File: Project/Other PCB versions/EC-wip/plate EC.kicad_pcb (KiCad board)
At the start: 4 copper layers, 245.7 x 83.6 mm, 154 parts, among them J2 USB_C_Receptacle_USB2.0, SW1 BOOT0, U1 USBLC6-2SC6, U2 XC6206PxxxMR-Regulator_Linear, U3 OPA354, U4 74AHCT1G125, U5 74HC4051, U7 74HC4051, U8 STM32F401CBUx, Y1 8 MHz

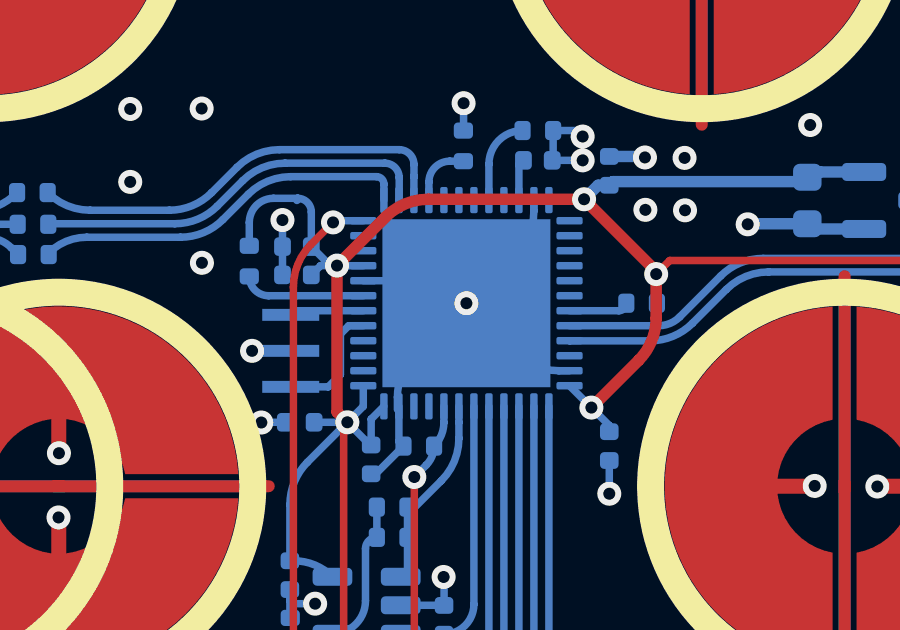
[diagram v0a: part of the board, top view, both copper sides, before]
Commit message: backup / cleanup
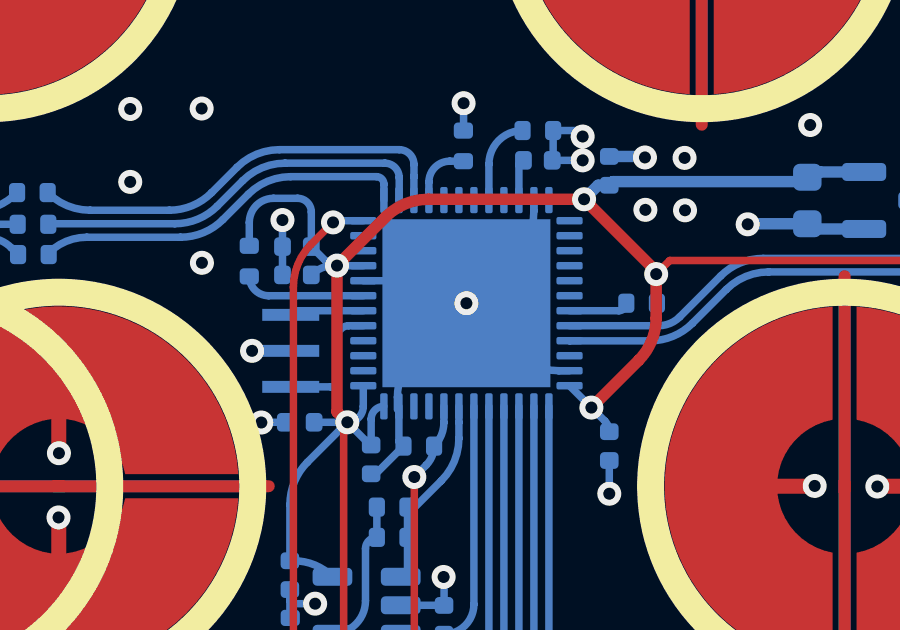
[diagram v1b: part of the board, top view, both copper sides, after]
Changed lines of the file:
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@@
     (fp_arc (start -47.899997 -1.516225) (mid -47.923178 -1.422766) (end -47.987348 -1.350973)
       (stroke (width 0.05) (type solid)) (layer "Dwgs.User"))
-    (fp_arc (start 47.899997 1.516225) (mid 47.923168 1.422757) (end 47.987348 1.350973)
+    (fp_arc (start 47.899997 1.516225) (mid 47.923176 1.422767) (end 47.987348 1.350973)
       (stroke (width 0.05) (type solid)) (layer "Dwgs.User"))
     (fp_arc (start 47.90625 8.616395) (mid 47.970705 8.522865) (end 48.081012 8.55)
@@
     (fp_arc (start 51.4 6.9) (mid 51.349937 6.898746) (end 51.3 6.894987)
       (stroke (width 0.05) (type solid)) (layer "Dwgs.User"))
-    (fp_arc (start 53.938297 8.040768) (mid 53.891169 7.945271) (end 53.875 7.840016)
+    (fp_arc (start 53.938297 8.040768) (mid 53.89117 7.945272) (end 53.875 7.840016)
       (stroke (width 0.05) (type solid)) (layer "Dwgs.User"))
-    (fp_arc (start 60.425 7.840016) (mid 60.408797 7.945261) (end 60.361703 8.040768)
+    (fp_arc (start 60.425 7.840016) (mid 60.408801 7.945264) (end 60.361703 8.040768)
       (stroke (width 0.05) (type solid)) (layer "Dwgs.User"))
     (fp_arc (start 63 6.894987) (mid 62.950063 6.898746) (end 62.9 6.9)
@@
     (fp_arc (start 66.312652 1.350973) (mid 66.376814 1.422772) (end 66.400003 1.516225)
       (stroke (width 0.05) (type solid)) (layer "Dwgs.User"))
-    (fp_arc (start 66.349999 8.533718) (mid 66.382117 8.569628) (end 66.39375 8.616395)
+    (fp_arc (start 66.349999 8.533718) (mid 66.382128 8.569633) (end 66.39375 8.616395)
       (stroke (width 0.05) (type solid)) (layer "Dwgs.User"))
     (fp_arc (start 66.35 9.100006) (mid 66.32071 9.170712) (end 66.250003 9.2)
@@
     (fp_arc (start 66.35 11.450023) (mid 66.247487 11.697487) (end 66.000023 11.8)
       (stroke (width 0.05) (type solid)) (layer "Dwgs.User"))
-    (fp_arc (start 66.400003 -1.516225) (mid 66.376832 -1.422757) (end 66.312652 -1.350973)
+    (fp_arc (start 66.400003 -1.516225) (mid 66.376824 -1.422767) (end 66.312652 -1.350973)
       (stroke (width 0.05) (type solid)) (layer "Dwgs.User"))
     (model "C:/Users/viva-/Documents/GitHub/libraries/cipulot_kicad_parts-main/cipulot_parts.3dshapes/Topre_OEM_Spacebar_7U.step"
@@
   (segment (start 105.819099 92.555) (end 105.840821 92.533278) (width 0.25) (layer "B.Cu") (net 19))
   (segment (start 51.28 51.183691) (end 51.28 52.3375) (width 0.25) (layer "B.Cu") (net 19))
-  (segment (start 61.2125 58.5075) (end 61.2125 58.3) (width 0.25) (layer "B.Cu") (net 19))
-  (segment (start 53.275 58.95125) (end 53.275 58.0875) (width 0.25) (layer "B.Cu") (net 19))
   (segment (start 61.333547 50.171453) (end 61.2125 50.2925) (width 0.381) (layer "B.Cu") (net 19))
   (segment (start 104.775 92.86875) (end 104.775 93.286014) (width 0.25) (layer "B.Cu") (net 19))
-  (segment (start 51.912929 52.970429) (end 51.28 52.3375) (width 0.25) (layer "B.Cu") (net 19))
   (segment (start 50.017837 50.727431) (end 50.82374 50.727431) (width 0.25) (layer "B.Cu") (net 19))
   (segment (start 62.8 54.225) (end 62.8 53.277946) (width 0.25) (layer "B.Cu") (net 19))
   (segment (start 67.813877 50.025808) (end 67.809287 50.030398) (width 0.381) (layer "B.Cu") (net 19))
   (segment (start 52.141254 52.975) (end 52.136683 52.970429) (width 0.25) (layer "B.Cu") (net 19))
-  (segment (start 52.136683 52.970429) (end 51.590821 52.970429) (width 0.25) (layer "B.Cu") (net 19))
-  (segment (start 53.0125 57.6625) (end 53.0125 56.975) (width 0.25) (layer "B.Cu") (net 19))
   (segment (start 104.775 92.555) (end 103.604726 92.555) (width 0.25) (layer "B.Cu") (net 19))
   (segment (start 67.46875 50.171453) (end 61.333547 50.171453) (width 0.381) (layer "B.Cu") (net 19))
-  (segment (start 61.2125 58.3) (end 60.616082 57.703582) (width 0.25) (layer "B.Cu") (net 19))
   (segment (start 50.566538 62.809503) (end 50.695502 62.809503) (width 0.25) (layer "B.Cu") (net 19))
   (segment (start 104.775 92.555) (end 105.819099 92.555) (width 0.25) (layer "B.Cu") (net 19))
@@
   (segment (start 103.604726 92.555) (end 103.6005 92.550774) (width 0.25) (layer "B.Cu") (net 19))
   (segment (start 60.3675 50.764327) (end 60.372179 50.759648) (width 0.25) (layer "B.Cu") (net 19))
+  (segment (start 51.754711 52.812211) (end 51.28 52.3375) (width 0.25) (layer "B.Cu") (net 19))
   (segment (start 50.566538 62.809503) (end 50.566538 60.936889) (width 0.25) (layer "B.Cu") (net 19))
-  (segment (start 53.275 58.0875) (end 53.7 57.6625) (width 0.25) (layer "B.Cu") (net 19))
+  (segment (start 53.0125 56.975) (end 53.0125 57.6625) (width 0.25) (layer "B.Cu") (net 19))
   (segment (start 51.37375 58.19375) (end 52.48125 58.19375) (width 0.25) (layer "B.Cu") (net 19))
+  (segment (start 60.616082 57.703582) (end 61.065775 58.153275) (width 0.25) (layer "B.Cu") (net 19))
   (segment (start 61.2125 50.2925) (end 60.839327 50.2925) (width 0.381) (layer "B.Cu") (net 19))
   (segment (start 60.3675 50.7875) (end 59.2 50.7875) (width 0.25) (layer "B.Cu") (net 19))
@@
   (segment (start 69.70625 49.85) (end 68.238315 49.85) (width 0.381) (layer "B.Cu") (net 19))
   (segment (start 60.839327 50.2925) (end 60.372179 50.759648) (width 0.381) (layer "B.Cu") (net 19))
-  (segment (start 51.590821 52.970429) (end 51.28 53.28125) (width 0.25) (layer "B.Cu") (net 19))
-  (segment (start 52.48125 58.19375) (end 53.0125 57.6625) (width 0.25) (layer "B.Cu") (net 19))
   (segment (start 60.616082 57.703582) (end 59.8875 56.975) (width 0.25) (layer "B.Cu") (net 19))
-  (segment (start 50.82374 50.727431) (end 50.82374 50.742687) (width 0.25) (layer "B.Cu") (net 19))
-  (segment (start 52.136683 52.970429) (end 51.912929 52.970429) (width 0.25) (layer "B.Cu") (net 19))
   (segment (start 62.8 53.277946) (end 62.7755 53.253446) (width 0.25) (layer "B.Cu") (net 19))
   (segment (start 52.48125 52.975) (end 53.0125 52.975) (width 0.25) (layer "B.Cu") (net 19))
@@
   (segment (start 187.833131 92.555) (end 188.9125 92.555) (width 0.25) (layer "B.Cu") (net 19))
   (segment (start 51.152325 59.522675) (end 52.48125 58.19375) (width 0.25) (layer "B.Cu") (net 19))
+  (segment (start 52.136683 52.970429) (end 52.030388 52.970429) (width 0.25) (layer "B.Cu") (net 19))
+  (segment (start 53.275 58.95125) (end 53.275 58.0875) (width 0.25) (layer "B.Cu") (net 19))
   (segment (start 53.275 58.95125) (end 53.23875 58.95125) (width 0.25) (layer "B.Cu") (net 19))
-  (arc (start 50.82374 50.742687) (mid 50.81757 50.773704) (end 50.8 50.8) (width 0.25) (layer "B.Cu") (net 19))
+  (arc (start 52.136683 52.970429) (mid 51.929961 52.929309) (end 51.754711 52.812211) (width 0.25) (layer "B.Cu") (net 19))
+  (arc (start 53.275 58.0875) (mid 53.39948 57.78698) (end 53.7 57.6625) (width 0.25) (layer "B.Cu") (net 19))
+  (arc (start 61.065775 58.153275) (mid 61.174367 58.315794) (end 61.2125 58.5075) (width 0.25) (layer "B.Cu") (net 19))
   (arc (start 188.9125 93.286014) (mid 188.964649 93.548189) (end 189.11316 93.77045) (width 0.25) (layer "B.Cu") (net 19))
   (arc (start 50.695502 62.809503) (mid 51.393529 62.948349) (end 51.985288 63.34375) (width 0.25) (layer "B.Cu") (net 19))
@@
   (arc (start 187.829597 92.556464) (mid 187.831218 92.555381) (end 187.833131 92.555) (width 0.25) (layer "B.Cu") (net 19))
   (arc (start 51.152325 59.522675) (mid 50.718779 60.171522) (end 50.566538 60.936889) (width 0.25) (layer "B.Cu") (net 19))
+  (arc (start 53.0125 57.6625) (mid 52.8569 58.03815) (end 52.48125 58.19375) (width 0.25) (layer "B.Cu") (net 19))
+  (arc (start 52.030388 52.970429) (mid 51.624281 53.051209) (end 51.28 53.28125) (width 0.25) (layer "B.Cu") (net 19))
   (arc (start 50.82374 50.727431) (mid 51.146365 50.861066) (end 51.28 51.183691) (width 0.25) (layer "B.Cu") (net 19))
   (arc (start 67.809287 50.030398) (mid 67.653047 50.134794) (end 67.46875 50.171453) (width 0.381) (layer "B.Cu") (net 19))
@@
   (segment (start 57.2 49.59) (end 57.2 50.7875) (width 0.25) (layer "B.Cu") (net 63))
   (arc (start 58.32125 48.46875) (mid 57.528407 48.797157) (end 57.2 49.59) (width 0.25) (layer "B.Cu") (net 63))
-  (segment (start 52.25 55.251992) (end 52.25 56.60625) (width 0.25) (layer "B.Cu") (net 67))
-  (segment (start 51.84375 57.0125) (end 50.59375 57.0125) (width 0.25) (layer "B.Cu") (net 67))
-  (segment (start 52.526992 54.975) (end 52.25 55.251992) (width 0.25) (layer "B.Cu") (net 67))
-  (segment (start 52.25 56.60625) (end 51.84375 57.0125) (width 0.25) (layer "B.Cu") (net 67))
+  (segment (start 50.59375 57.0125) (end 51.935508 57.0125) (width 0.25) (layer "B.Cu") (net 67))
+  (segment (start 52.162201 56.785807) (end 52.162201 55.339791) (width 0.25) (layer "B.Cu") (net 67))
   (segment (start 53.0125 54.975) (end 52.526992 54.975) (width 0.25) (layer "B.Cu") (net 67))
+  (arc (start 52.162201 55.339791) (mid 52.269046 55.081845) (end 52.526992 54.975) (width 0.25) (layer "B.Cu") (net 67))
+  (arc (start 51.935508 57.0125) (mid 52.095804 56.946103) (end 52.162201 56.785807) (width 0.25) (layer "B.Cu") (net 67))
   (segment (start 53.0125 54.475) (end 50.73125 54.475) (width 0.25) (layer "B.Cu") (net 68))
-  (segment (start 50.73125 54.475) (end 50.59375 54.6125) (width 0.25) (layer "B.Cu") (net 68))
+  (arc (start 50.73125 54.475) (mid 50.634023 54.515273) (end 50.59375 54.6125) (width 0.25) (layer "B.Cu") (net 68))
   (segment (start 56.349625 49.490642) (end 55.893323 49.490642) (width 0.25) (layer "B.Cu") (net 71))
   (segment (start 55.2 50.7875) (end 55.2 50.183965) (width 0.25) (layer "B.Cu") (net 71))
